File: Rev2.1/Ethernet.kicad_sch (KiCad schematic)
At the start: 33 parts, among them J13 8P8C_LED, T1 H1102NLT, U12 USBLC6-4SC6, U8 LAN8742A, Y3 25Mhz

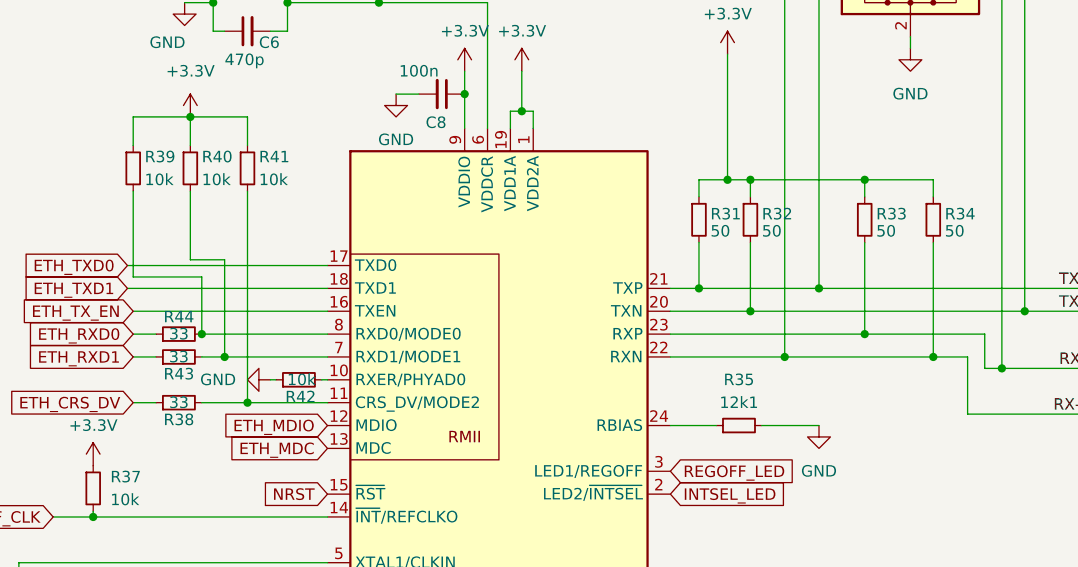
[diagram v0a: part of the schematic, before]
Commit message: done about 2/3 of the routing for the board
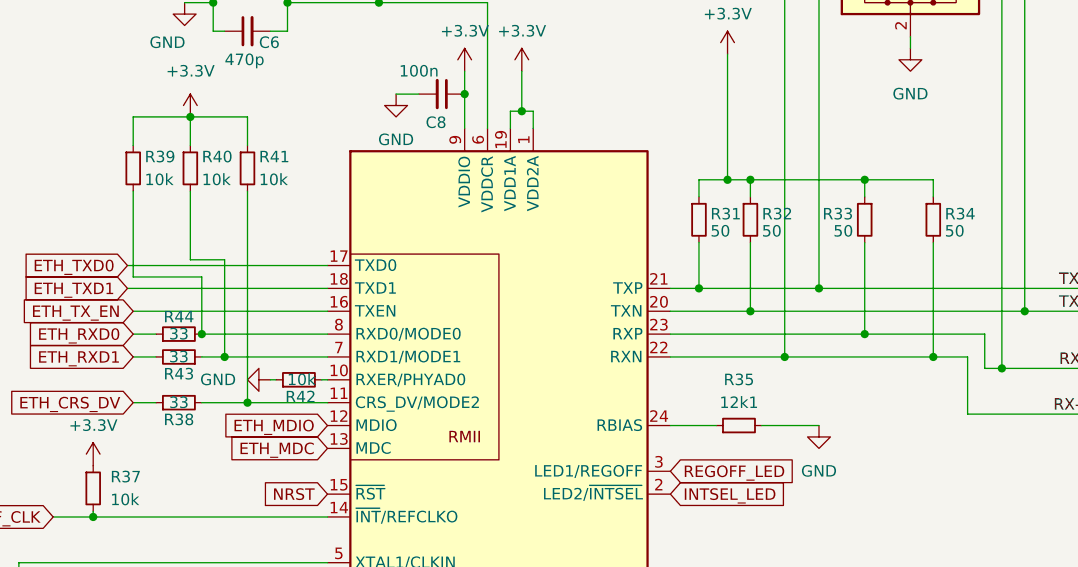
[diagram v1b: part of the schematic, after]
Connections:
- net ETH_RXD1: now also R43.2; no longer R43.1
- net at R40.2, U8.7 (RXD1/MODE1): now also R43.1; no longer R43.2
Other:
- moved on the sheet: R43
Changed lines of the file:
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@@
     )
   )
-  (symbol (lib_id "Device:R_Small") (at 144.78 86.36 0) (unit 1)
-    (in_bom yes) (on_board yes) (dnp no)
-    (property "Reference" "R33" (at 146.05 85.725 0)
-      (effects (font (size 1.27 1.27)) (justify left))
-    )
-    (property "Value" "50" (at 146.05 87.63 0)
+  (symbol (lib_id "Device:R_Small") (at 144.78 86.36 0) (mirror y) (unit 1)
+    (in_bom yes) (on_board yes) (dnp no)
+    (property "Reference" "R33" (at 143.51 85.725 0)
+      (effects (font (size 1.27 1.27)) (justify left))
+    )
+    (property "Value" "50" (at 143.51 87.63 0)
       (effects (font (size 1.27 1.27)) (justify left))
     )
@@
     )
   )
-  (symbol (lib_id "Device:R_Small") (at 68.58 101.6 90) (unit 1)
+  (symbol (lib_id "Device:R_Small") (at 68.58 101.6 270) (mirror x) (unit 1)
     (in_bom yes) (on_board yes) (dnp no)
     (property "Reference" "R43" (at 68.58 103.505 90)
